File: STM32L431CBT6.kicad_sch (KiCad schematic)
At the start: 20 parts, among them J1 SWD, SW1 Reset, U1 STM32L431CBTx, Y1 8M

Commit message: purge shit
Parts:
- C11, C12, C13, C14, C15, C16, C17, C21, C22, C7: footprint Capacitor_SMD:C_0805_2012Metric -> (none)
- CR1, CR2: footprint UTSVT_ICs:SOT26_DIO -> (none)
- FB1, FB4: footprint Inductor_SMD:L_0805_2012Metric -> (none)
- J1: footprint Connector_PinHeader_2.54mm:PinHeader_1x04_P2.54mm_Vertical -> (none)
- R19, R29: footprint Resistor_SMD:R_0805_2012Metric -> (none)
- SW1: footprint Button_Switch_SMD:SW_SPST_B3SL-1002P -> (none)
- U1: footprint Package_QFP:LQFP-48_7x7mm_P0.5mm -> (none)
- Y1: footprint Crystal:Crystal_SMD_TXC_7A-2Pin_5x3.2mm -> (none)
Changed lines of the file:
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@@
 			)
 		)
-		(property "Footprint" "UTSVT_ICs:SOT26_DIO"
+		(property "Footprint" ""
 			(at 218.44 127 0)
 			(effects
@@
 			)
 		)
-		(property "Footprint" "Capacitor_SMD:C_0805_2012Metric"
+		(property "Footprint" ""
 			(at 100.0252 186.69 0)
 			(effects
@@
 			)
 		)
-		(property "Footprint" "Capacitor_SMD:C_0805_2012Metric"
+		(property "Footprint" ""
 			(at 115.2652 151.13 0)
 			(effects
@@
 			)
 		)
-		(property "Footprint" "Button_Switch_SMD:SW_SPST_B3SL-1002P"
+		(property "Footprint" ""
 			(at 115.57 182.88 0)
 			(effects
@@
 			)
 		)
-		(property "Footprint" "Capacitor_SMD:C_0805_2012Metric"
+		(property "Footprint" ""
 			(at 79.7052 151.13 0)
 			(effects
@@
 			)
 		)
-		(property "Footprint" "Inductor_SMD:L_0805_2012Metric"
+		(property "Footprint" ""
 			(at 55.88 182.118 90)
 			(effects
@@
 			)
 		)
-		(property "Footprint" "Capacitor_SMD:C_0805_2012Metric"
+		(property "Footprint" ""
 			(at 61.9252 187.96 0)
 			(effects
@@
 			)
 		)
-		(property "Footprint" "Capacitor_SMD:C_0805_2012Metric"
+		(property "Footprint" ""
 			(at 100.0252 151.13 0)
 			(effects
@@
 			)
 		)
-		(property "Footprint" "Resistor_SMD:R_0805_2012Metric"
+		(property "Footprint" ""
 			(at 110.998 50.8 90)
 			(effects
@@
 			)
 		)
-		(property "Footprint" "UTSVT_ICs:SOT26_DIO"
+		(property "Footprint" ""
 			(at 219.71 101.6 0)
 			(effects
@@
 			)
 		)
-		(property "Footprint" "Capacitor_SMD:C_0805_2012Metric"
+		(property "Footprint" ""
 			(at 67.0052 151.13 0)
 			(effects
@@
 			)
 		)
-		(property "Footprint" "Capacitor_SMD:C_0805_2012Metric"
+		(property "Footprint" ""
 			(at 88.9 39.0652 0)
 			(effects
@@
 			)
 		)
-		(property "Footprint" "Capacitor_SMD:C_0805_2012Metric"
+		(property "Footprint" ""
 			(at 55.5752 151.13 0)
 			(effects
@@
 			)
 		)
-		(property "Footprint" "Crystal:Crystal_SMD_TXC_7A-2Pin_5x3.2mm"
+		(property "Footprint" ""
 			(at 101.6 43.18 0)
 			(effects
@@
 			)
 		)
-		(property "Footprint" "Inductor_SMD:L_0805_2012Metric"
+		(property "Footprint" ""
 			(at 140.335 122.428 90)
 			(effects
@@
 			)
 		)
-		(property "Footprint" "Connector_PinHeader_2.54mm:PinHeader_1x04_P2.54mm_Vertical"
+		(property "Footprint" ""
 			(at 144.78 144.78 0)
 			(effects
@@
 			)
 		)
-		(property "Footprint" "Capacitor_SMD:C_0805_2012Metric"
+		(property "Footprint" ""
 			(at 88.9 49.2252 0)
 			(effects
@@
 			)
 		)
-		(property "Footprint" "Resistor_SMD:R_0805_2012Metric"
+		(property "Footprint" ""
 			(at 107.442 171.45 90)
 			(effects
@@
 			)
 		)
-		(property "Footprint" "Capacitor_SMD:C_0805_2012Metric"
+		(property "Footprint" ""
 			(at 44.1452 151.13 0)
 			(effects
@@
 			)
 		)
-		(property "Footprint" "Package_QFP:LQFP-48_7x7mm_P0.5mm"
+		(property "Footprint" ""
 			(at 128.27 105.41 0)
 			(effects

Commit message: initial PP changes
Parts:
- C11, C12, C14, C15, C16, C17, C7: P/N C0805C104M5RACTU -> (none)
- C13: P/N GRM219R6YA475KA73D -> (none)
- C21, C22: P/N C0805C120K5HACTU -> (none)
- CR1, CR2: P/N D5V0P4UR6SO-7 -> (none)
- R19: P/N CRCW08051K00FKEAC -> (none)
- R29: P/N CRCW080510K0FKEAC -> (none)
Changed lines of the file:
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@@
 			)
 		)
-		(property "P/N" "D5V0P4UR6SO-7"
+		(property "P/N" ""
 			(at 198.12 130.81 0)
 			(effects
@@
 			)
 		)
-		(property "P/N" "C0805C104M5RACTU"
+		(property "P/N" ""
 			(at 99.06 182.88 0)
 			(effects
@@
 			)
 		)
-		(property "P/N" "C0805C104M5RACTU"
+		(property "P/N" ""
 			(at 114.3 147.32 0)
 			(effects
@@
 			)
 		)
-		(property "P/N" "C0805C104M5RACTU"
+		(property "P/N" ""
 			(at 78.74 147.32 0)
 			(effects
@@
 			)
 		)
-		(property "P/N" "C0805C104M5RACTU"
+		(property "P/N" ""
 			(at 60.96 184.15 0)
 			(effects
@@
 			)
 		)
-		(property "P/N" "C0805C104M5RACTU"
+		(property "P/N" ""
 			(at 99.06 147.32 0)
 			(effects
@@
 			)
 		)
-		(property "P/N" "CRCW08051K00FKEAC"
+		(property "P/N" ""
 			(at 109.22 50.8 0)
 			(effects
@@
 			)
 		)
-		(property "P/N" "D5V0P4UR6SO-7"
+		(property "P/N" ""
 			(at 199.39 105.41 0)
 			(effects
@@
 			)
 		)
-		(property "P/N" "C0805C104M5RACTU"
+		(property "P/N" ""
 			(at 66.04 147.32 0)
 			(effects
@@
 			)
 		)
-		(property "P/N" "C0805C120K5HACTU"
+		(property "P/N" ""
 			(at 92.71 38.1 0)
 			(effects
@@
 			)
 		)
-		(property "P/N" "C0805C104M5RACTU"
+		(property "P/N" ""
 			(at 54.61 147.32 0)
 			(effects
@@
 			)
 		)
-		(property "P/N" "C0805C120K5HACTU"
+		(property "P/N" ""
 			(at 92.71 48.26 0)
 			(effects
@@
 			)
 		)
-		(property "P/N" "CRCW080510K0FKEAC"
+		(property "P/N" ""
 			(at 109.22 171.45 0)
 			(effects
@@
 			)
 		)
-		(property "P/N" "GRM219R6YA475KA73D"
+		(property "P/N" ""
 			(at 43.18 147.32 0)
 			(effects

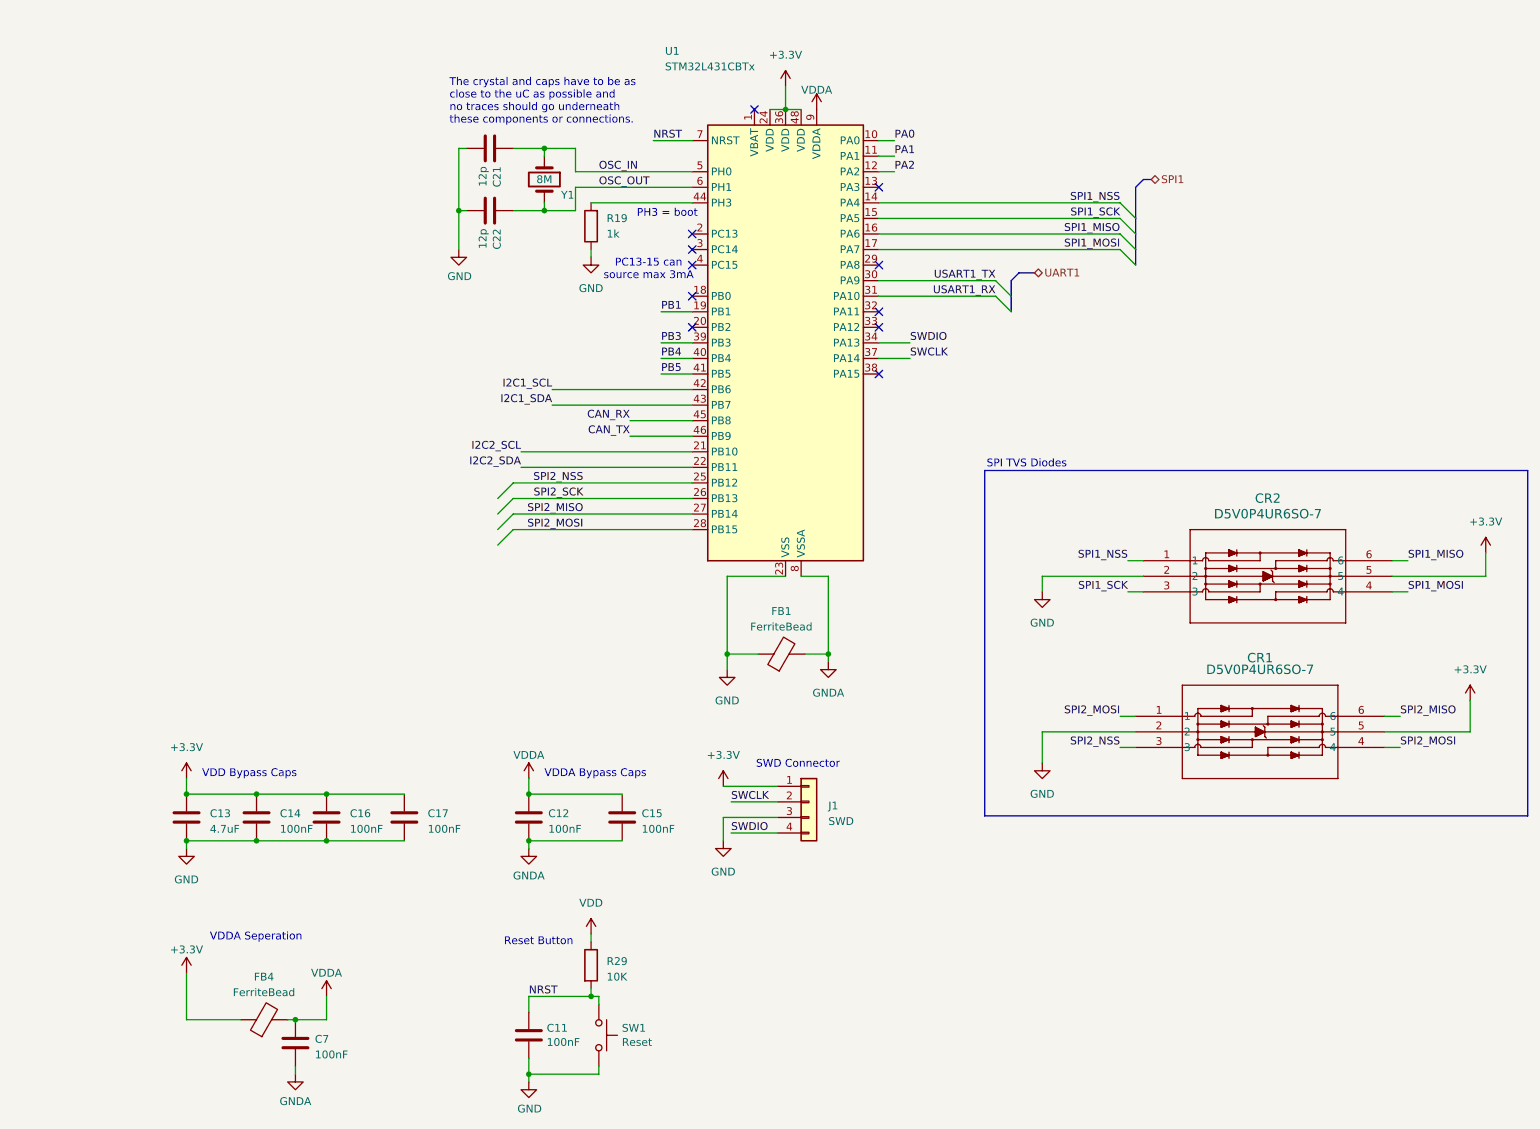
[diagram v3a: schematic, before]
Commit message: stuf
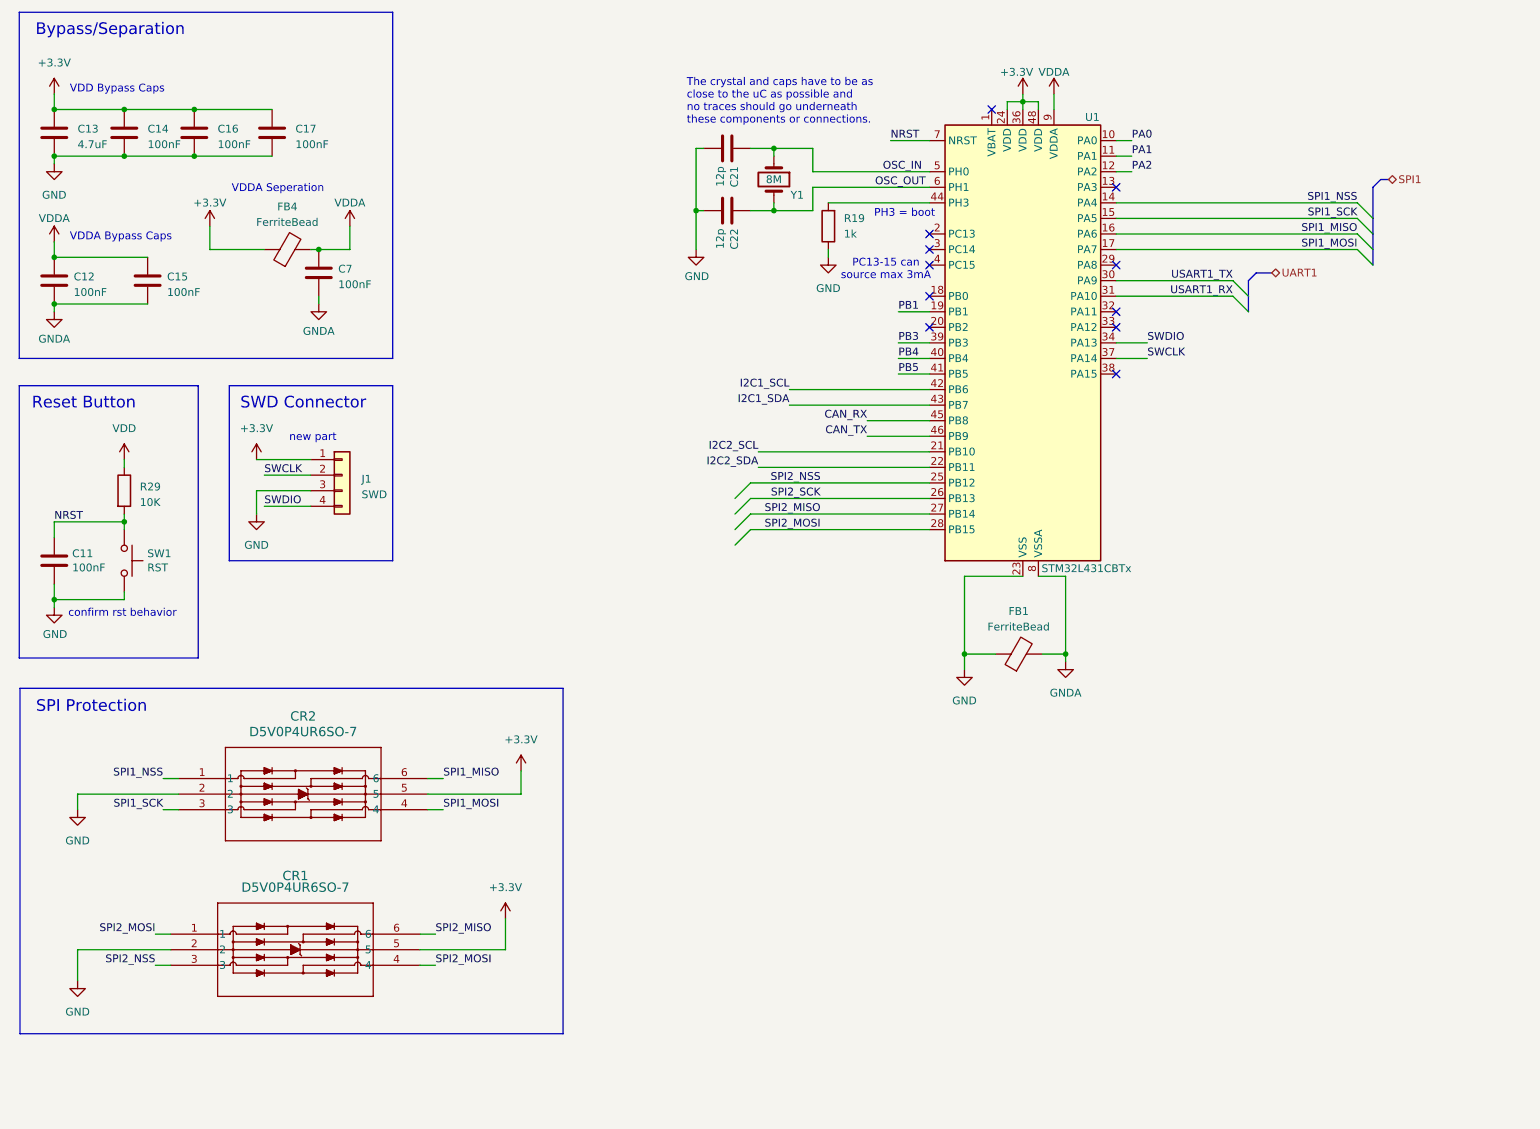
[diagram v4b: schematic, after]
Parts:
- SW1: value Reset -> RST
- U1: footprint (none) -> Package_QFP:LQFP-48_7x7mm_P0.5mm
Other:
- note added: "Bypass/Separation"
- note added: "SPI Protection"
- note added: "confirm rst behavior"
- note added: "new part"
- note removed: "SPI TVS Diodes"
- title: (none) -> MCU
- moved on the sheet: C11, C12, C13, C14, C15, C16, C17, C21, C22, C7, CR1, CR2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
